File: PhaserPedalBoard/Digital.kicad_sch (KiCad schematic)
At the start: 37 parts, among them J1 Footswitch, J2 SWD Header, Q1 BC847, Q2 2N7002, Q3 2N7002, Q7 2N7002, SW2 RST, U6 STM32L052K6T6, U7 LM2904

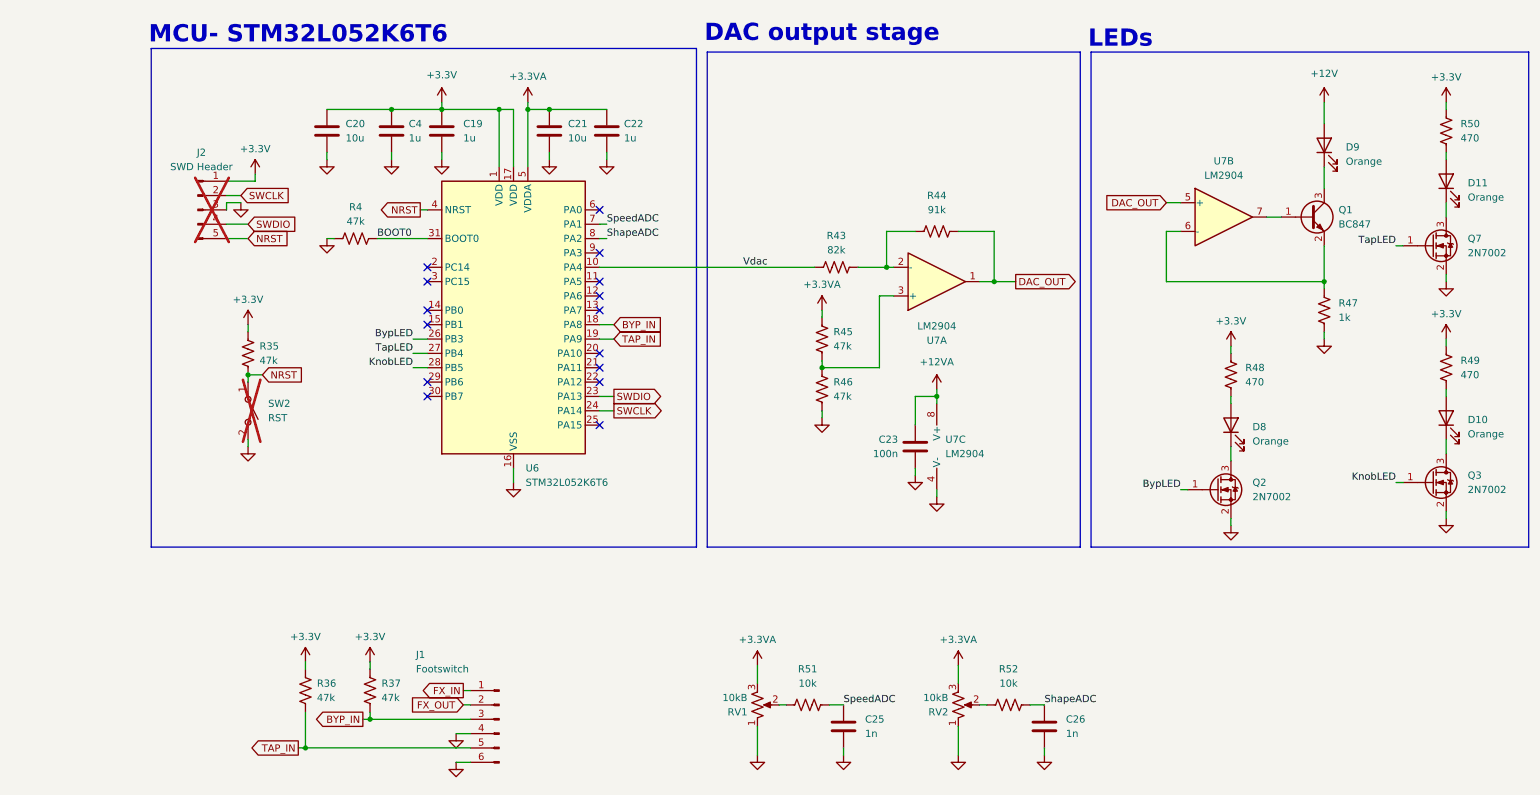
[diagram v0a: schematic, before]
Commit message: schematic hygiene
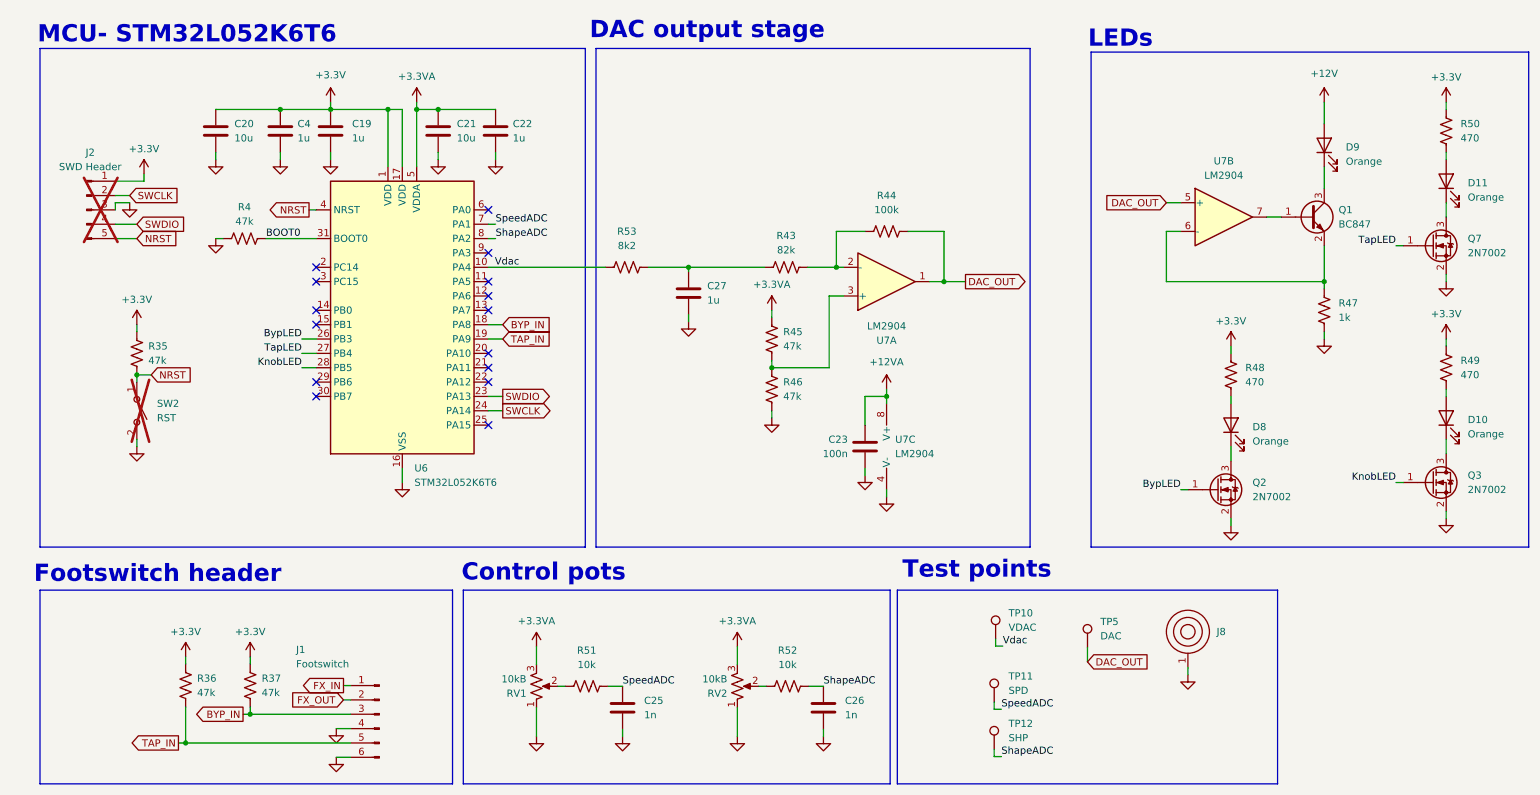
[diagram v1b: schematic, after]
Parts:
- added C27: 1u, symbol Device:C
- added J8: (no value), Connector:BatteryContact_Keystone_243, symbol Connector:GroundingSpring
- added R53: 8k2, symbol Device:R_US
- added TP10: VDAC, TestPoint:TestPoint_THTPad_D2.0mm_Drill1.0mm_VAL, symbol Connector:TestPoint
- added TP11: SPD, TestPoint:TestPoint_THTPad_D2.0mm_Drill1.0mm_VAL, symbol Connector:TestPoint
- added TP12: SHP, TestPoint:TestPoint_THTPad_D2.0mm_Drill1.0mm_VAL, symbol Connector:TestPoint
- added TP5: DAC, TestPoint:TestPoint_THTPad_D2.0mm_Drill1.0mm_VAL, symbol Connector:TestPoint
- R44: value 91k -> 100k
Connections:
- net DAC_OUT: now also TP5.1
- net GND: now also C27.2, J8.1
- net ShapeADC: now also TP12.1
- net SpeedADC: now also TP11.1
- net Vdac: now also R53.1, TP10.1; no longer R43.1
- new net: C27.1, R43.1, R53.2
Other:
- note added: "Control pots"
- note added: "Footswitch header"
- note added: "Test points"
- moved on the sheet: C19, C20, C21, C22, C23, C25, C26, C4, J1, J2, R35, R36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
